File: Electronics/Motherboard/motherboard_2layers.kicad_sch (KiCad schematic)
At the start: 54 parts, among them J1 DX07S024JJ3R1300, J2 Conn_02x10_Odd_Even, M1 AO3400A, M2 AO3400A, M3 AO3400A, U1 AMS1117-3.3, U2 TMC2209_SILENTSTEPSTICK, U3 TMC2209_SILENTSTEPSTICK, U4 TMC2209_SILENTSTEPSTICK, U5 TMC2209_SILENTSTEPSTICK, U6 LM2576HVS-5, U8 STM32F405RGTx

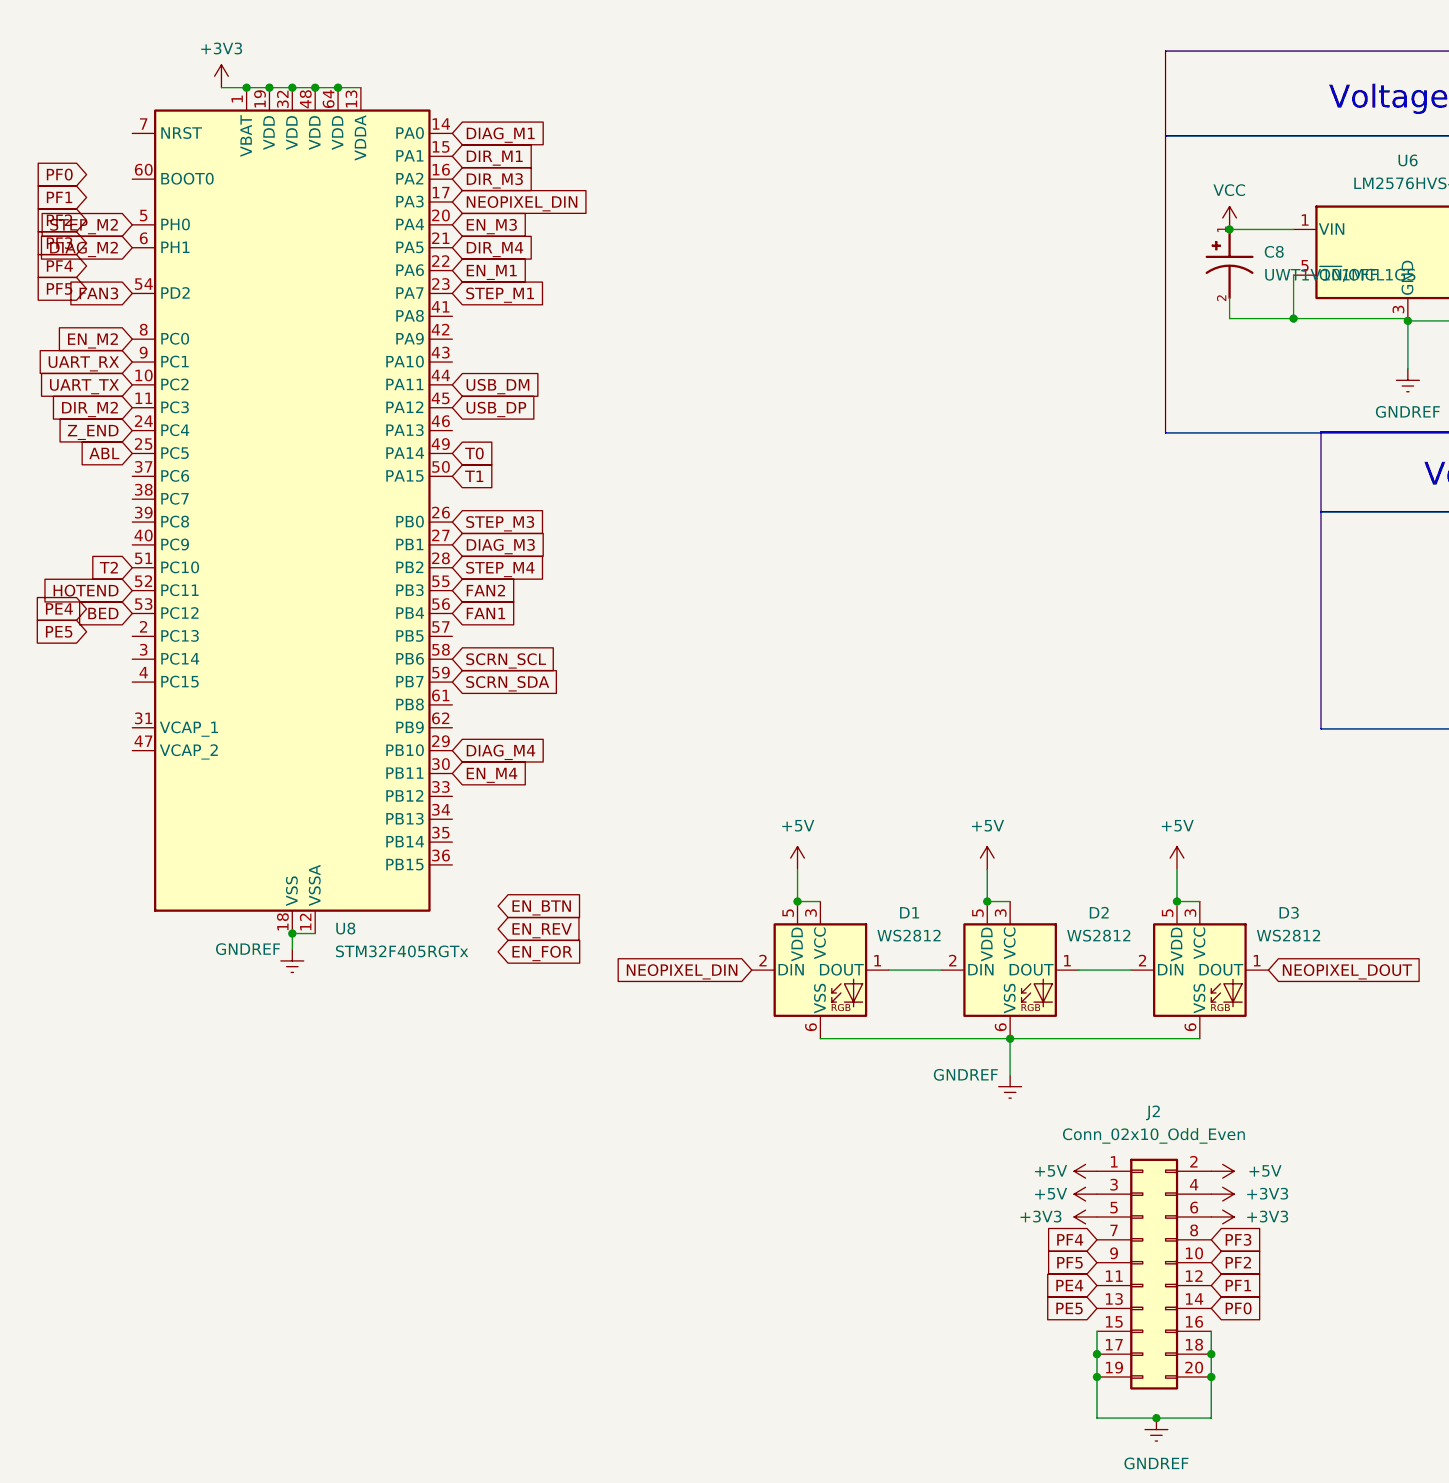
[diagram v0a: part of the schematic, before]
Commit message: tiny bit of routing, more needs to be done
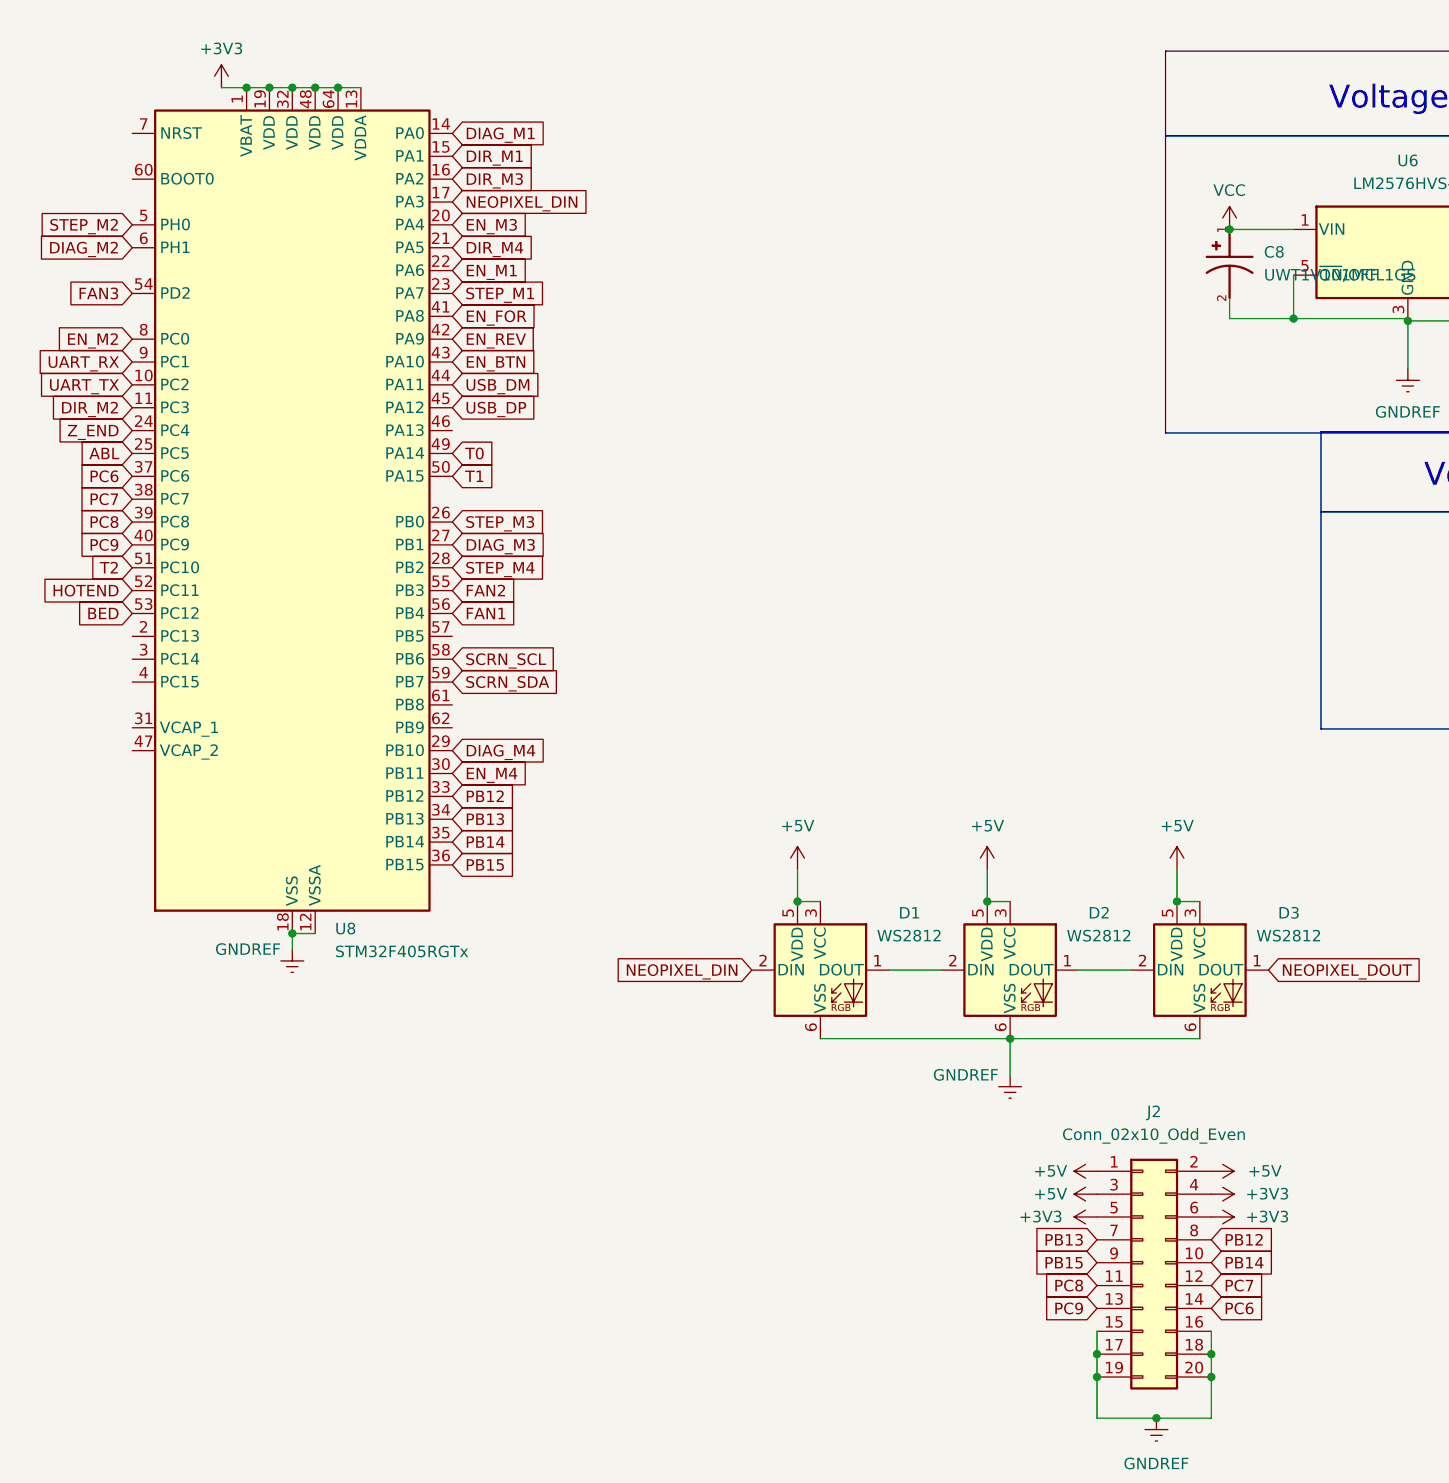
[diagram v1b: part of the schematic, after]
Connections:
- net PE4 is gone; now on net PC8: J2.11 (Pin_11)
- net PE5 is gone; now on net PC9: J2.13 (Pin_13)
- net PF0 is gone; now on net PC6: J2.14 (Pin_14)
- net PF1 is gone; now on net PC7: J2.12 (Pin_12)
- net PF2 is gone; now on net PB14: J2.10 (Pin_10)
- net PF3 is gone; now on net PB12: J2.8 (Pin_8)
- net PF4 is gone; now on net PB13: J2.7 (Pin_7)
- net PF5 is gone; now on net PB15: J2.9 (Pin_9)
- net EN_BTN: now also U8.43 (PA10)
- net EN_FOR: now also U8.41 (PA8)
- net EN_REV: now also U8.42 (PA9)
- net PB12: now reaches U8.33 (PB12)
- net PB13: now reaches U8.34 (PB13)
- net PB14: now reaches U8.35 (PB14)
- net PB15: now reaches U8.36 (PB15)
- net PC6: now reaches U8.37 (PC6)
- net PC7: now reaches U8.38 (PC7)
- net PC8: now reaches U8.39 (PC8)
- net PC9: now reaches U8.40 (PC9)
